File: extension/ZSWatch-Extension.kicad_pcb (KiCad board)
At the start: 4 copper layers, 45 x 36.9 mm, 37 parts, among them IC501 DA7212-01UM2, IC502 MAX32664, IC503 MAX86141, IC504 LIS2DS12, X501 MB1, X502 MB2, Y501 32kHz

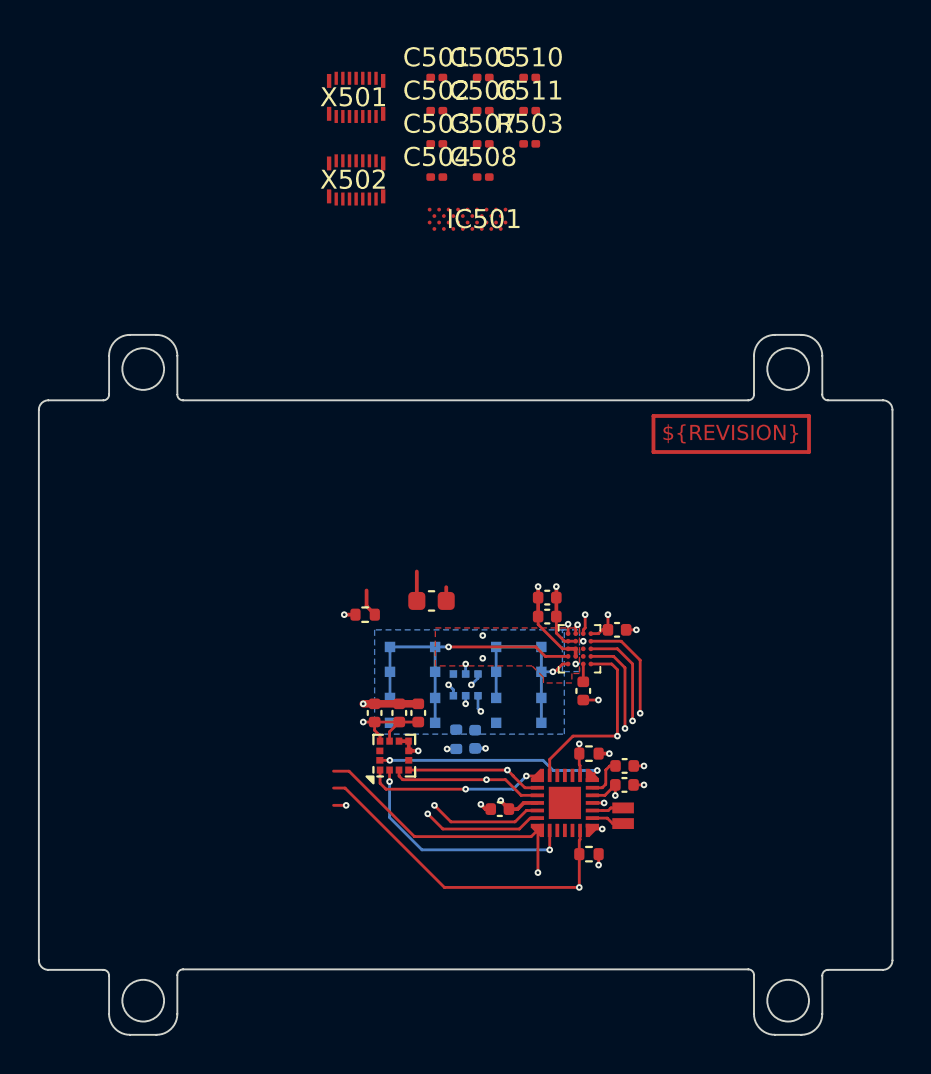
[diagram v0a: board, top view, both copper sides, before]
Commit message: First version done
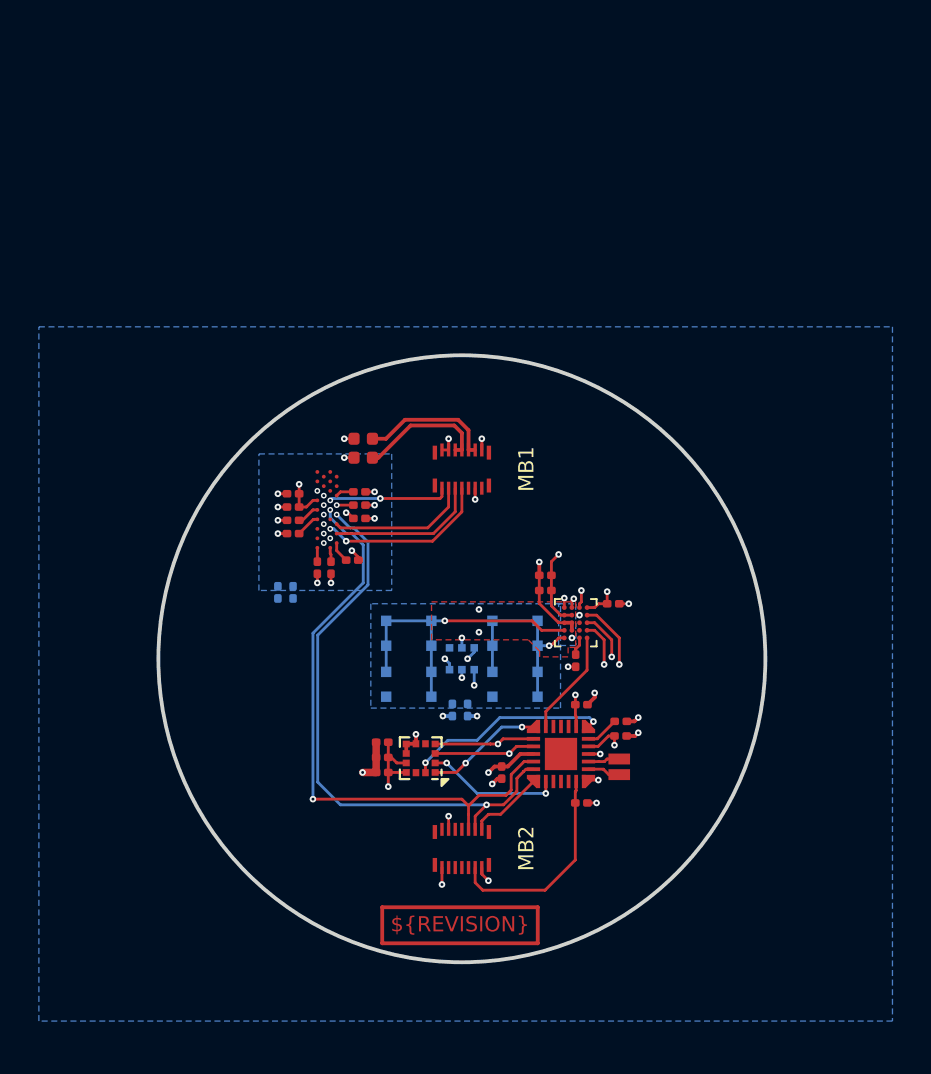
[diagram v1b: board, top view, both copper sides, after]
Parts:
- removed C402: 1u, Capacitor_SMD:C_0603_1608Metric
- removed R407: 10k, Resistor_SMD:R_0402_1005Metric
- added C522: 100n, Capacitor_SMD:C_0201_0603Metric, B.Cu at (196.1, 146.5)
- added FB501: FerriteBead, Inductor_SMD:L_0402_1005Metric, F.Cu at (199.8, 139.4)
- added FB502: FerriteBead, Inductor_SMD:L_0402_1005Metric, F.Cu at (199.8, 138.4)
- C509, C512, C513, C514, C515, C516, C517, C518, C519, C520, C521: footprint Capacitor_SMD:C_0402_1005Metric -> Capacitor_SMD:C_0201_0603Metric
- R501, R504: footprint Resistor_SMD:R_0402_1005Metric -> Resistor_SMD:R_0201_0603Metric
- R502: footprint Resistor_SMD:R_0402_1005Metric -> Inductor_SMD:L_0201_0603Metric
- R503: value R_Small -> 0R; moved to B.Cu
- moved X502 35.7 mm to (205.0, 160.0)
- moved C510 27.9 mm to (198.1, 145.2), turned to -90 degrees
- moved R503 27.1 mm to (195.3, 146.5), turned to 90 degrees
- moved C511 26.6 mm to (197.4, 145.2), turned to -90 degrees
- moved C505 23.5 mm to (199.6, 141.9)
- moved C506 22.5 mm to (196.1, 141.3), turned to 180 degrees
- moved C501 22.2 mm to (199.6, 141.2)
- moved C502 21.9 mm to (199.6, 142.6)
- moved C507 21.6 mm to (196.1, 142.0), turned to 180 degrees
- moved C508 21.3 mm to (199.2, 144.8)
- moved C503 21.2 mm to (196.1, 142.7), turned to 180 degrees
- moved X501 20.4 mm to (205.0, 140.0)
- moved C504 20.3 mm to (196.1, 143.4), turned to 180 degrees
- moved IC501 17.0 mm to (197.9, 142.2), turned to 90 degrees
- moved C519 3.16 mm to (200.8, 156.0), turned to 180 degrees
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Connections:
- X501 pad 1: /Project Architecture/Main/I2S_DIN -> /Project Architecture/Main/I2S_MCLK
- X501 pad 10: unconnected-(X501-Pin_10-Pad10) -> /Project Architecture/Main/SP-N
- X501 pad 11: /Project Architecture/Main/SP-P -> +1V8
- X501 pad 12: /Project Architecture/Main/SP-P -> /Project Architecture/Main/SP-N
- X501 pad 13: /Project Architecture/Main/SP-N -> unconnected-(X501-Pin_13-Pad13)
- X501 pad 14: /Project Architecture/Main/SP-N -> GND
- X501 pad 2: /Project Architecture/Main/I2S_BCLK -> GND
- X501 pad 4: /Project Architecture/Main/I2S_MCLK -> GND
- X501 pad 5: unconnected-(X501-Pin_5-Pad5) -> /Project Architecture/Main/I2S_BCLK
- X501 pad 6: unconnected-(X501-Pin_6-Pad6) -> /Project Architecture/Main/SP-P
- X501 pad 7: GND -> /Project Architecture/Main/I2S_DIN
- X501 pad 8: unconnected-(X501-Pin_8-Pad8) -> /Project Architecture/Main/SP-P
- X502 pad 1: +1V8 -> VSYS
- X502 pad 10: /Project Architecture/Main/~{RESET_{HR}} -> /Project Architecture/Main/SDA
- X502 pad 11: /Project Architecture/Main/STATUS -> /Project Architecture/Main/~{RESET_{HR}}
- X502 pad 12: unconnected-(X502-Pin_12-Pad12) -> /Project Architecture/Main/SCL
- X502 pad 13: unconnected-(X502-Pin_13-Pad13) -> GND
- X502 pad 14: GND -> /Project Architecture/Main/STATUS
- X502 pad 2: VSYS -> unconnected-(X502-Pin_2-Pad2)
- X502 pad 3: V_{DD} -> unconnected-(X502-Pin_3-Pad3)
- X502 pad 4: unconnected-(X502-Pin_4-Pad4) -> V_{DD}
- X502 pad 8: /Project Architecture/Main/SDA -> unconnected-(X502-Pin_8-Pad8)
- X502 pad 9: /Project Architecture/Main/SCL -> unconnected-(X502-Pin_9-Pad9)
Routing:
- net /Project Architecture/Main/SDA: track 11.4 -> 31.7 mm
- net /Project Architecture/Main/SCL: track 12.0 -> 30.7 mm, vias 1 -> 2
- net /Project Architecture/Main/STATUS: track 14.6 -> 4.22 mm, vias 1 -> 0
- net /Project Architecture/Main/I2S_DIN: track 0.00 -> 9.10 mm, vias 0 -> 2
- net /Project Architecture/Main/I2S_BCLK: track 0.00 -> 7.97 mm
- net /Project Architecture/Main/I2S_WCLK: track 0.00 -> 7.43 mm
- net /Project Architecture/Main/SP-N: track 0.00 -> 7.10 mm
- net /Project Architecture/Main/~{RESET_{HR}}: track 18.1 -> 11.1 mm, vias 1 -> 0
- net /Project Architecture/Main/SP-P: track 0.00 -> 6.83 mm
- net /Project Architecture/Main/I2S_MCLK: track 0.00 -> 6.42 mm, vias 0 -> 2
- net Net-(IC502-CS_{ACC}): track 12.7 -> 7.13 mm
- net Net-(IC502-MISO_{SENSOR}): track 22.5 -> 17.4 mm
- net Net-(IC502-CS_{PPG}): track 9.95 -> 5.57 mm, vias 1 -> 0
- net GNDA: track 0.00 -> 4.32 mm, vias 0 -> 12
- net Net-(IC502-SCLK_{SENSOR}): track 26.1 -> 21.8 mm
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- added copper zone on B.Cu, net GND
- added copper zone on B.Cu, net GNDA
- added copper zone on In1.Cu, net V_{DD}
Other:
- board size 45 x 36.9 mm -> 32 x 32 mm
